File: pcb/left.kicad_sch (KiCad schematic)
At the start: 56 parts, among them J1 USB_C_Receptacle_PowerOnly_6P, SW1 SW_Push, SW10 SW_Push, SW11 SW_Push, SW12 SW_Push, SW13 SW_Push, SW14 SW_Push, SW15 SW_Push, SW16 SW_Push, SW17 SW_Push, SW18 SW_Push, SW19 SW_Push, SW2 SW_Push, SW20 SW_Push, SW21 SW_Push, SW22 SW_Push, SW23 SW_Push, SW3 SW_Push, SW4 SW_Push, SW5 SW_Push, SW6 SW_Push, SW7 SW_Push, SW8 SW_Push, SW9 SW_Push, U1 ProMicro

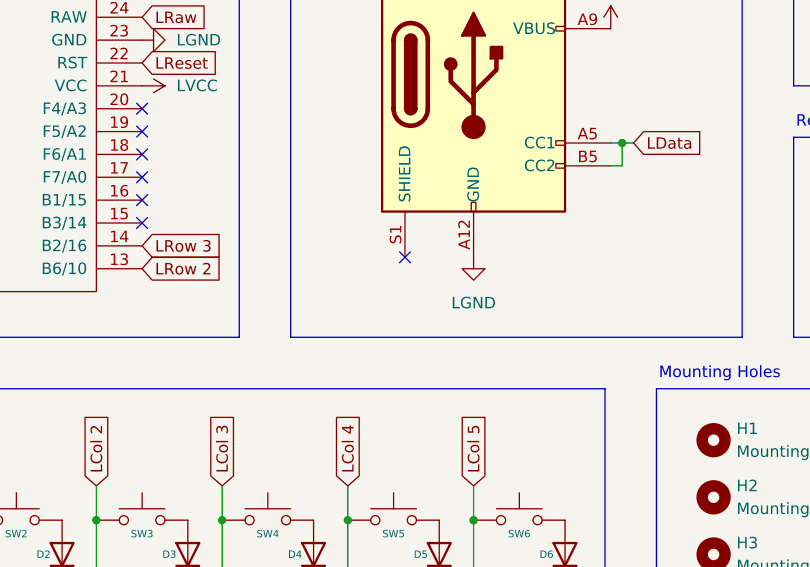
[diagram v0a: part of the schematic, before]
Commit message: docs: add bill of materials
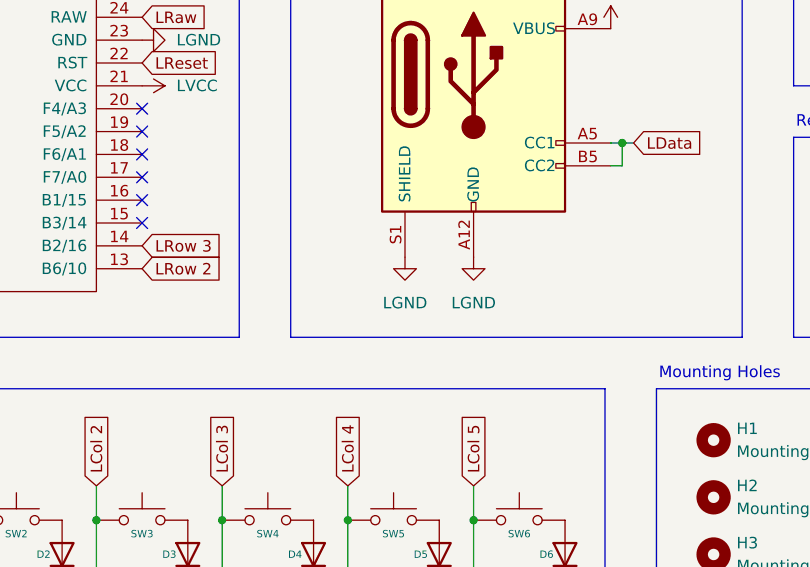
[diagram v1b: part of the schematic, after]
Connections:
- net LGND: now also J1.S1 (SHIELD)
- no-connect marks 8 -> 7
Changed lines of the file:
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@@
 	)
 	(no_connect
-		(at 93.98 58.42)
-	)
-	(no_connect
 		(at 64.77 54.61)
 	)
@@
 					(unit 1)
 				)
+			)
+		)
+	)
+	(symbol
+		(lib_id "power:GND")
+		(at 93.98 58.42 0)
+		(unit 1)
+		(exclude_from_sim no)
+		(in_bom yes)
+		(on_board yes)
+		(dnp no)
+		(property "Reference" "#PWR021"
+			(at 93.98 64.77 0)
+			(effects
+				(font
+					(size 1.27 1.27)
+				)
+				(hide yes)
+			)
+		)
+		(property "Value" "LGND"
+			(at 93.98 63.5 0)
+			(effects
+				(font
+					(size 1.27 1.27)
+				)
+			)
+		)
+		(property "Footprint" ""
+			(at 93.98 58.42 0)
+			(effects
+				(font
+					(size 1.27 1.27)
+				)
+				(hide yes)
+			)
+		)
+		(property "Datasheet" ""
+			(at 93.98 58.42 0)
+			(effects
+				(font
+					(size 1.27 1.27)
+				)
+				(hide yes)
+			)
+		)
+		(property "Description" "Power symbol creates a global label with name \"GND\" , ground"
+			(at 93.98 58.42 0)
+			(effects
+				(font
+					(size 1.27 1.27)
+				)
+				(hide yes)
+			)
+		)
+		(pin "1"
+		)
+		(instances
+			(project "Flake"
+				(path "/90c8b5ef-2115-4ce5-9f08-3facf16c5dc1/56cc3e7f-98ec-487b-8cea-9eac8504bc25"
+					(reference "#PWR021")
+					(unit 1)
+				)

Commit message: pcb: smd controller footprint
use smd prom-micro footprint
easier to break off the last column
wider controller cutout
ground usb shield
reroute some paths
minimse a chance of damaging the pcb after brakeing off the pinky column
edit silkscreen
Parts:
- U1: footprint axseem:ProMicro -> axseem:ProMicro_SMD
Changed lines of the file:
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@@
 			)
 		)
-		(property "Footprint" "axseem:ProMicro"
+		(property "Footprint" "axseem:ProMicro_SMD"
 			(at 49.53 72.39 0)
 			(effects

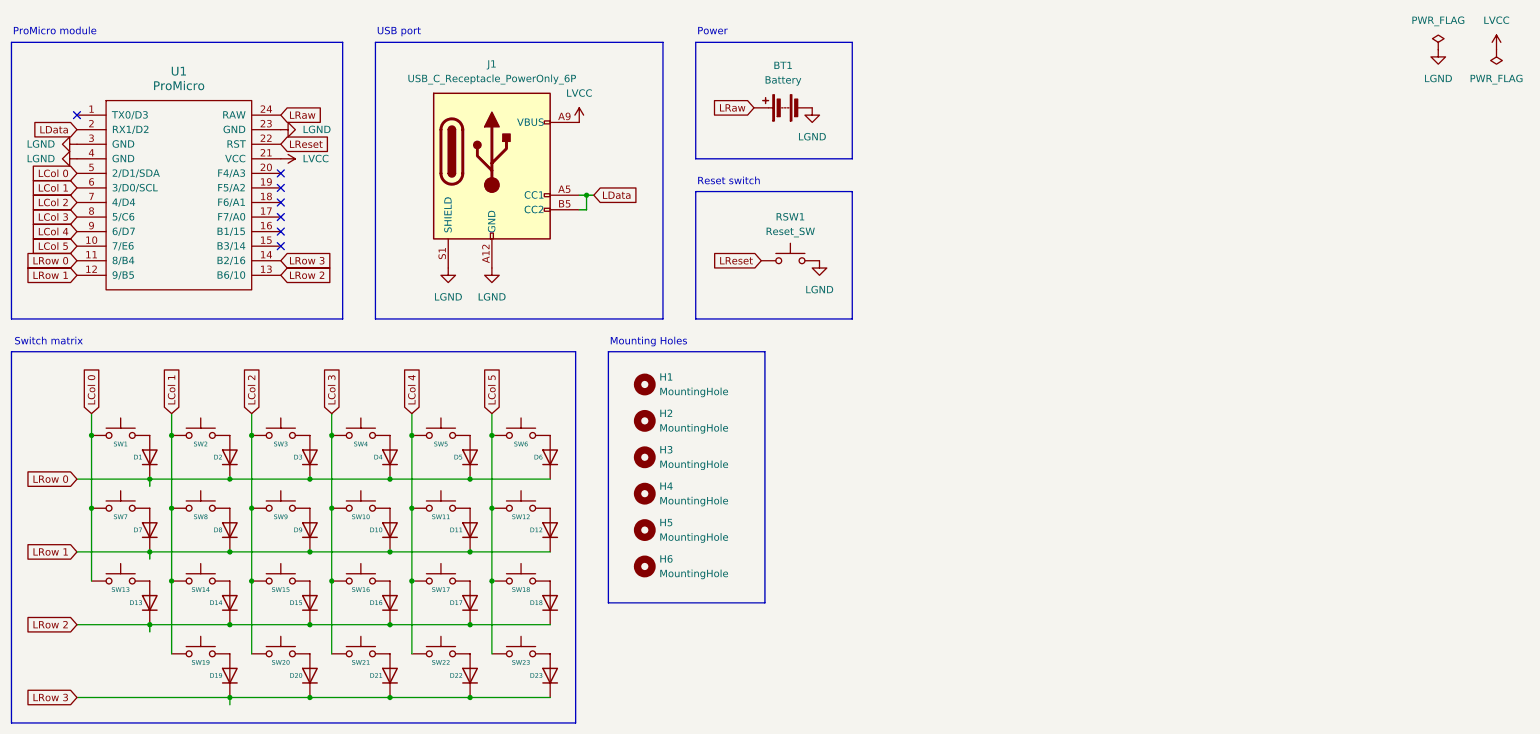
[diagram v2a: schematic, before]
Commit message: updates
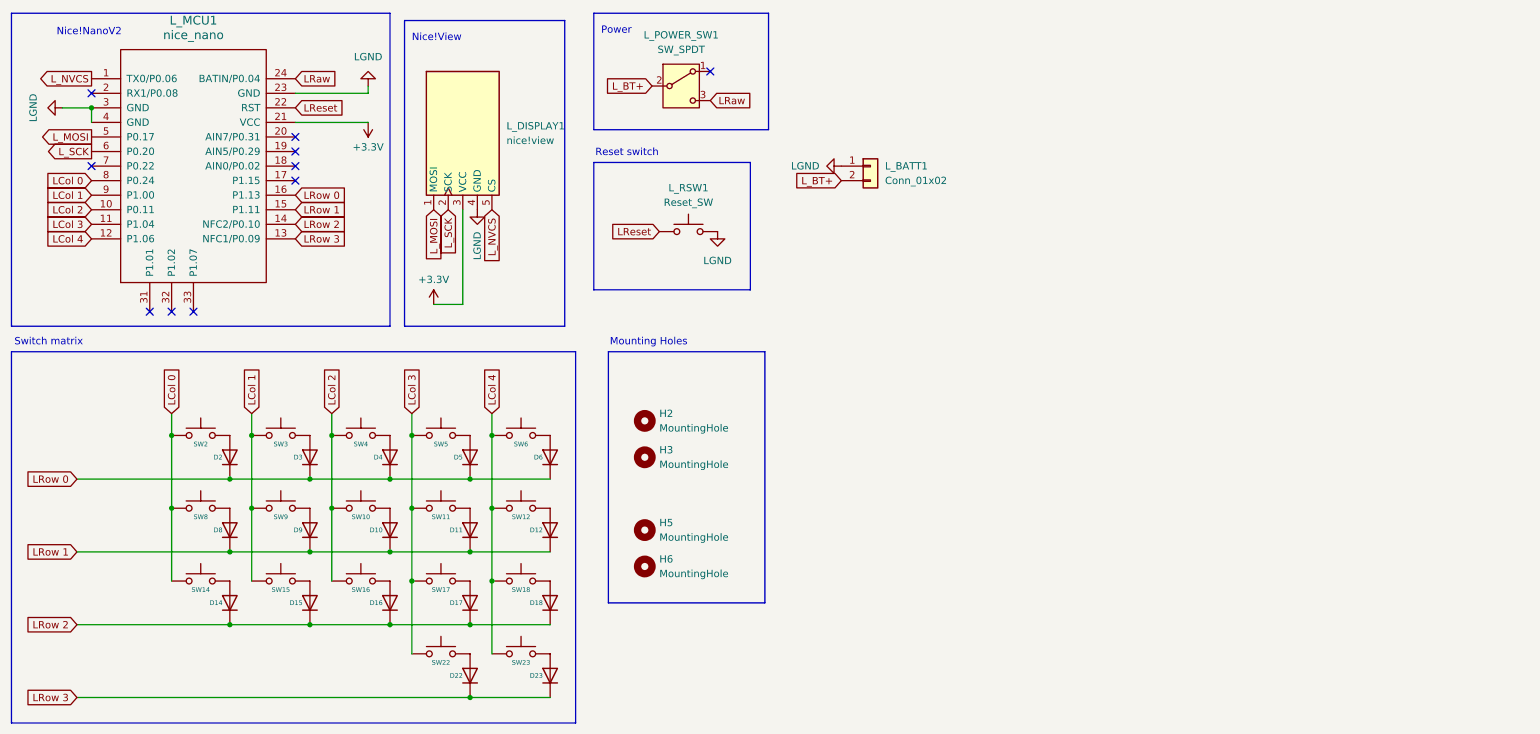
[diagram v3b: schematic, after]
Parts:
- removed BT1: Battery, axseem:JST_1.25mm_mid-mount, symbol Device:Battery
- removed D1, D13, D19, D20, D21, D7: D, axseem:D_SOD-123_Handsoldering, symbol Device:D
- removed H1, H4: MountingHole, MountingHole:MountingHole_2.2mm_M2, symbol Mechanical:MountingHole
- removed J1: USB_C_Receptacle_PowerOnly_6P, axseem:USB-C_6Pin_Mid-mount, symbol Connector:USB_C_Receptacle_PowerOnly_6P
- removed SW1, SW13, SW19, SW20, SW21, SW7: SW_Push, axseem:SW_MX_Choc-v1v2_Hotswap, symbol Switch:SW_Push
- removed U1: ProMicro, axseem:ProMicro_SMD, symbol kbd:ProMicro
- added L_BATT1: Conn_01x02, Connector_JST:JST_PH_S2B-PH-K_1x02_P2.00mm_Horizontal, symbol Connector_Generic:Conn_01x02
- added L_DISPLAY1: nice!view, axseem:nice_view, symbol nice_nano:nice!view
- added L_MCU1: nice_nano, axseem:nice_nano, symbol nice_nano:nice_nano
- added L_POWER_SW1: SW_SPDT, axseem:smt-slider-switch, symbol Switch:SW_SPDT
- L_RSW1: renamed from RSW1; footprint axseem:TS-1289VE-4 -> axseem:SMD_RESET
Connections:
- net LCol 5 is gone; now on net LCol 4: SW12.1, SW18.1, SW23.1, SW6.1
- net LCol 0: now also SW14.1, SW2.1, SW8.1, L_MCU1.8 (P0.24)
- net LCol 1: now also SW15.1, SW3.1, SW9.1, L_MCU1.9 (P1.00); no longer SW14.1, SW2.1, SW8.1
- net LCol 2: now also SW10.1, SW16.1, SW4.1, L_MCU1.10 (P0.11); no longer SW15.1, SW3.1, SW9.1
- net LCol 3: now also SW11.1, SW17.1, SW22.1, SW5.1, L_MCU1.11 (P1.04); no longer SW10.1, SW16.1, SW4.1
- net LCol 4: now also L_MCU1.12 (P1.06); no longer SW11.1, SW17.1, SW22.1, SW5.1
- net LGND: now also L_BATT1.1 (Pin_1), L_DISPLAY1.4 (GND), L_MCU1.23 (GND), L_MCU1.3 (GND), L_MCU1.4 (GND)
- net LRaw: now also L_MCU1.24 (BATIN/P0.04), L_POWER_SW1.3 (C)
- net LReset: now also L_MCU1.22 (RST)
- net LRow 0: now also L_MCU1.16 (P1.13)
- net LRow 1: now also L_MCU1.15 (P1.11)
- net LRow 2: now also L_MCU1.14 (NFC2/P0.10)
- net LRow 3: now also L_MCU1.13 (NFC1/P0.09)
- new net +3.3V: L_DISPLAY1.3 (VCC), L_MCU1.21 (VCC)
- new net L_BT+: L_BATT1.2 (Pin_2), L_POWER_SW1.2 (B)
- new net L_MOSI: L_DISPLAY1.1 (MOSI), L_MCU1.5 (P0.17)
- new net L_NVCS: L_DISPLAY1.5 (CS), L_MCU1.1 (TX0/P0.06)
- new net L_SCK: L_DISPLAY1.2 (SCK), L_MCU1.6 (P0.20)
- no-connect marks 7 -> 10
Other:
- note added: "Nice!NanoV2"
- note added: "Nice!View"
- note removed: "ProMicro module"
- note removed: "USB port"
- moved on the sheet: L_RSW1

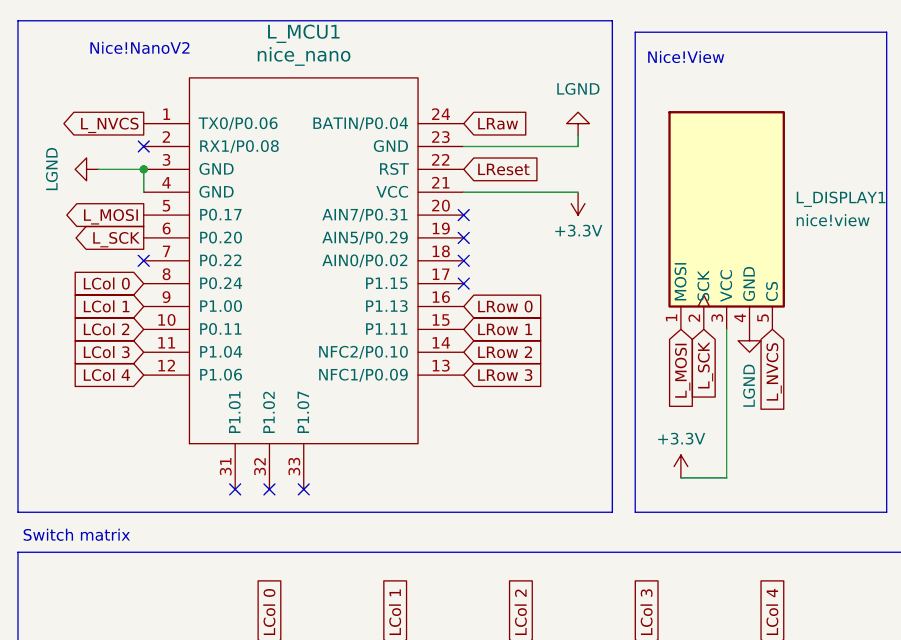
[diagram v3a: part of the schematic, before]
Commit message: update
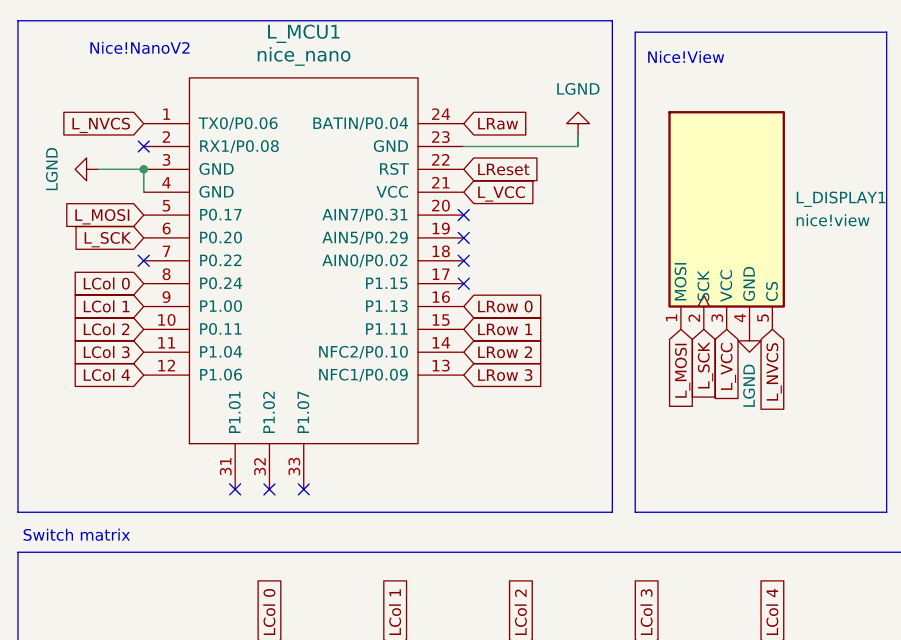
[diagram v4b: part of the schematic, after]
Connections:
- net +3.3V renamed L_VCC
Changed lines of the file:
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@@
 	(wire
 		(pts
-			(xy 96.52 64.77) (xy 96.52 48.26)
-		)
-		(stroke
-			(width 0)
-			(type default)
-		)
-	)
-	(wire
-		(pts
 			(xy 55.88 95.25) (xy 69.85 95.25)
 		)
@@
 	(wire
 		(pts
-			(xy 67.31 33.02) (xy 80.01 33.02)
-		)
-		(stroke
-			(width 0)
-			(type default)
-		)
-	)
-	(wire
-		(pts
 			(xy 69.85 95.25) (xy 83.82 95.25)
 		)
@@
 	(wire
 		(pts
-			(xy 91.44 64.77) (xy 96.52 64.77)
-		)
-		(stroke
-			(width 0)
-			(type default)
-		)
-	)
-	(wire
-		(pts
 			(xy 87.63 87.63) (xy 87.63 100.33)
 		)
@@
 		)
 	)
+	(global_label "L_VCC"
+		(shape input)
+		(at 96.52 48.26 270)
+		(fields_autoplaced yes)
+		(effects
+			(font
+				(size 1.27 1.27)
+			)
+			(justify right)
+		)
+		(property "Intersheetrefs" "${INTERSHEET_REFS}"
+			(at 96.52 56.8695 90)
+			(effects
+				(font
+					(size 1.27 1.27)
+				)
+				(justify right)
+				(hide yes)
+			)
+		)
+	)
 	(global_label "LRow 2"
 		(shape input)
@@
 	)
 	(global_label "L_MOSI"
-		(shape output)
+		(shape input)
 		(at 31.75 35.56 180)
 		(fields_autoplaced yes)
@@
 	)
 	(global_label "L_SCK"
-		(shape output)
+		(shape input)
 		(at 31.75 38.1 180)
 		(fields_autoplaced yes)
@@
 		)
 	)
+	(global_label "L_VCC"
+		(shape input)
+		(at 67.31 33.02 0)
+		(fields_autoplaced yes)
+		(effects
+			(font
+				(size 1.27 1.27)
+			)
+			(justify left)
+		)
+		(property "Intersheetrefs" "${INTERSHEET_REFS}"
+			(at 75.9195 33.02 0)
+			(effects
+				(font
+					(size 1.27 1.27)
+				)
+				(justify left)
+				(hide yes)
+			)
+		)
+	)
 	(global_label "LCol 1"
 		(shape input)
@@
 	)
 	(global_label "L_NVCS"
-		(shape output)
+		(shape input)
 		(at 31.75 25.4 180)
 		(fields_autoplaced yes)
@@
 	)
 	(symbol
-		(lib_id "power:+3.3V")
-		(at 80.01 33.02 180)
-		(unit 1)
-		(exclude_from_sim no)
-		(in_bom yes)
-		(on_board yes)
-		(dnp no)
-		(property "Reference" "#PWR015"
-			(at 80.01 29.21 0)
-			(effects
-				(font
-					(size 1.27 1.27)
-				)
-				(hide yes)
-			)
-		)
-		(property "Value" "+3.3V"
-			(at 80.01 37.338 0)
-			(effects
-				(font
-					(size 1.27 1.27)
-				)
-			)
-		)
-		(property "Footprint" ""
-			(at 80.01 33.02 0)
-			(effects
-				(font
-					(size 1.27 1.27)
-				)
-				(hide yes)
-			)
-		)
-		(property "Datasheet" ""
-			(at 80.01 33.02 0)
-			(effects
-				(font
-					(size 1.27 1.27)
-				)
-				(hide yes)
-			)
-		)
-		(property "Description" "Power symbol creates a global label with name \"+3.3V\""
-			(at 80.01 33.02 0)
-			(effects
-				(font
-					(size 1.27 1.27)
-				)
-				(hide yes)
-			)
-		)
-		(pin "1"
-		)
-		(instances
-			(project "Flake"
-				(path "/90c8b5ef-2115-4ce5-9f08-3facf16c5dc1/56cc3e7f-98ec-487b-8cea-9eac8504bc25"
-					(reference "#PWR015")
-					(unit 1)
-				)
-			)
-		)
-	)
-	(symbol
 		(lib_id "Switch:SW_Push")
 		(at 50.8 87.63 0)
@@
 					(unit 1)
 				)
-			)
-		)
-	)
-	(symbol
-		(lib_id "power:+3.3V")
-		(at 91.44 64.77 0)
-		(unit 1)
-		(exclude_from_sim no)
-		(in_bom yes)
-		(on_board yes)
-		(dnp no)
-		(property "Reference" "#PWR010"
-			(at 91.44 68.58 0)
-			(effects
-				(font
-					(size 1.27 1.27)
-				)
-				(hide yes)
-			)
-		)
-		(property "Value" "+3.3V"
-			(at 91.44 60.452 0)
-			(effects
-				(font
-					(size 1.27 1.27)
-				)
-			)
-		)
-		(property "Footprint" ""
-			(at 91.44 64.77 0)
-			(effects
-				(font
-					(size 1.27 1.27)
-				)
-				(hide yes)
-			)
-		)
-		(property "Datasheet" ""
-			(at 91.44 64.77 0)
-			(effects
-				(font
-					(size 1.27 1.27)
-				)
-				(hide yes)
-			)
-		)
-		(property "Description" "Power symbol creates a global label with name \"+3.3V\""
-			(at 91.44 64.77 0)
-			(effects
-				(font
-					(size 1.27 1.27)
-				)
-				(hide yes)
-			)
-		)
-		(pin "1"
-		)
-		(instances
-			(project ""
-				(path "/90c8b5ef-2115-4ce5-9f08-3facf16c5dc1/56cc3e7f-98ec-487b-8cea-9eac8504bc25"
-					(reference "#PWR010")
-					(unit 1)
-				)
